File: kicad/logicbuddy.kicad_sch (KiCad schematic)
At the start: 33 parts, among them J1 USB_C_2PIN, Q1 NPN, Q2 NPN, Q3 NPN, Q4 NPN, Q5 NPN, Q6 NPN, Q7 NPN, SW1 SW_SPST, SW2 SW_SPST, SW3 SW_SPST, SW4 SW_SPST, SW5 SW_SPST, SW6 SW_SPST, SW7 SW_SPST, SW8 SW_DIP_x01

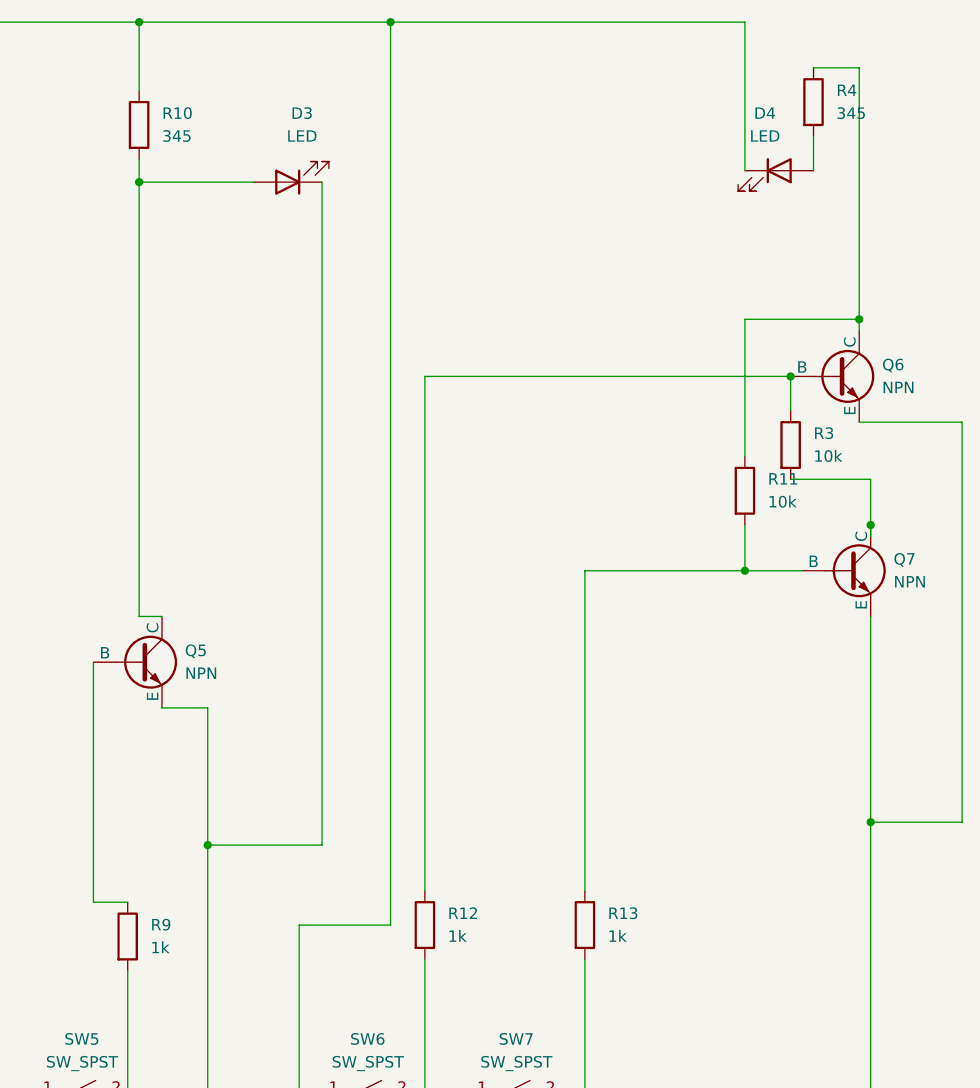
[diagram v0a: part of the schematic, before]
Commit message: Reapply "updated labels and fixed footprints"
This reverts commit 2a946a7896d612220efc5a586cb72ca7f3163489.
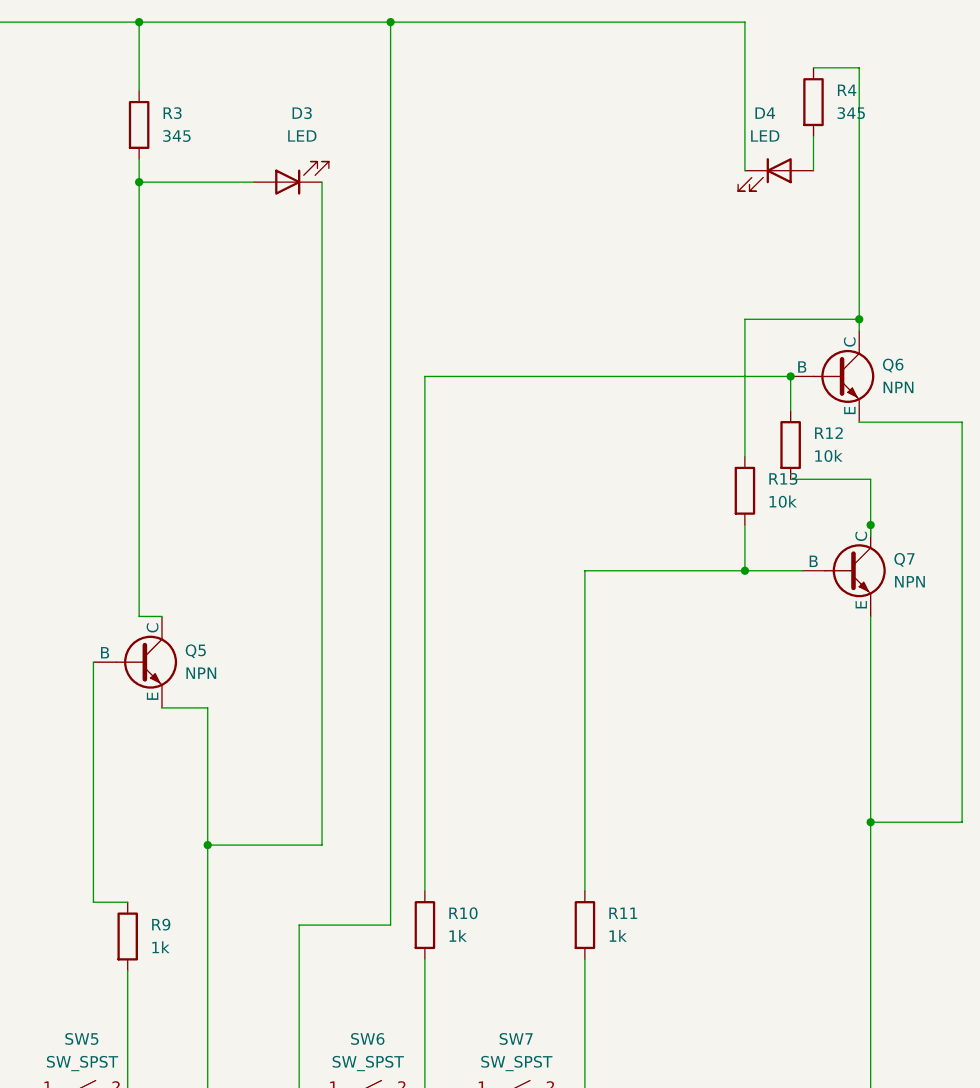
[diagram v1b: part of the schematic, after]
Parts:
- J1: footprint Connector_USB:USB_C_Receptacle_G-Switch_GT-USB-7010ASV -> Aliexpress crap:USB_C_2pin-aliexpress
- SW1, SW2, SW3, SW4, SW5, SW6, SW7: footprint Button_Switch_THT:SW_Push_2P1T_Toggle_CK_PVA1xxH1xxxxxxV2 -> Button_Switch_THT:SW_PUSH_6mm_H5mm
- renumbered R12 to R10, R13 to R11, R3 to R12, R11 to R13, R10 to R3
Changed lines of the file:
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@@
 			)
 		)
-		(property "Footprint" "Button_Switch_THT:SW_Push_2P1T_Toggle_CK_PVA1xxH1xxxxxxV2"
+		(property "Footprint" "Button_Switch_THT:SW_PUSH_6mm_H5mm"
 			(at 92.71 140.97 0)
 			(effects
@@
 			)
 		)
-		(property "Footprint" "Button_Switch_THT:SW_Push_2P1T_Toggle_CK_PVA1xxH1xxxxxxV2"
+		(property "Footprint" "Button_Switch_THT:SW_PUSH_6mm_H5mm"
 			(at 118.11 140.97 0)
 			(effects
@@
 		(dnp no)
 		(fields_autoplaced yes)
-		(property "Reference" "R3"
+		(property "Reference" "R12"
 			(at 234.95 67.3099 0)
 			(effects
@@
 			(project ""
 				(path "/3781676b-6fe7-418a-9d16-7dd26fe4a4bc"
-					(reference "R3")
+					(reference "R12")
 					(unit 1)
 				)
@@
 		(dnp no)
 		(fields_autoplaced yes)
-		(property "Reference" "R12"
+		(property "Reference" "R10"
 			(at 194.31 120.6499 0)
 			(effects
@@
 			(project ""
 				(path "/3781676b-6fe7-418a-9d16-7dd26fe4a4bc"
-					(reference "R12")
+					(reference "R10")
 					(unit 1)
 				)
@@
 			)
 		)
-		(property "Footprint" "Button_Switch_THT:SW_Push_2P1T_Toggle_CK_PVA1xxH1xxxxxxV2"
+		(property "Footprint" "Button_Switch_THT:SW_PUSH_6mm_H5mm"
 			(at 63.5 142.24 0)
 			(effects
@@
 			)
 		)
-		(property "Footprint" "Connector_USB:USB_C_Receptacle_G-Switch_GT-USB-7010ASV"
+		(property "Footprint" "Aliexpress crap:USB_C_2pin-aliexpress"
 			(at 53.34 171.45 0)
 			(effects
@@
 			)
 		)
-		(property "Footprint" "Button_Switch_THT:SW_Push_2P1T_Toggle_CK_PVA1xxH1xxxxxxV2"
+		(property "Footprint" "Button_Switch_THT:SW_PUSH_6mm_H5mm"
 			(at 36.83 142.24 0)
 			(effects
@@
 			)
 		)
-		(property "Footprint" "Button_Switch_THT:SW_Push_2P1T_Toggle_CK_PVA1xxH1xxxxxxV2"
+		(property "Footprint" "Button_Switch_THT:SW_PUSH_6mm_H5mm"
 			(at 201.93 140.97 0)
 			(effects
@@
 			)
 		)
-		(property "Footprint" "Button_Switch_THT:SW_Push_2P1T_Toggle_CK_PVA1xxH1xxxxxxV2"
+		(property "Footprint" "Button_Switch_THT:SW_PUSH_6mm_H5mm"
 			(at 185.42 140.97 0)
 			(effects
@@
 		(dnp no)
 		(fields_autoplaced yes)
-		(property "Reference" "R11"
+		(property "Reference" "R13"
 			(at 229.87 72.3899 0)
 			(effects
@@
 			(project ""
 				(path "/3781676b-6fe7-418a-9d16-7dd26fe4a4bc"
-					(reference "R11")
+					(reference "R13")
 					(unit 1)
 				)
@@
 		(dnp no)
 		(fields_autoplaced yes)
-		(property "Reference" "R10"
+		(property "Reference" "R3"
 			(at 162.56 31.7499 0)
 			(effects
@@
 			(project ""
 				(path "/3781676b-6fe7-418a-9d16-7dd26fe4a4bc"
-					(reference "R10")
+					(reference "R3")
 					(unit 1)
 				)
@@
 		(dnp no)
 		(fields_autoplaced yes)
-		(property "Reference" "R13"
+		(property "Reference" "R11"
 			(at 212.09 120.6499 0)
 			(effects
@@
 			(project ""
 				(path "/3781676b-6fe7-418a-9d16-7dd26fe4a4bc"
-					(reference "R13")
+					(reference "R11")
 					(unit 1)
 				)
@@
 			)
 		)
-		(property "Footprint" "Button_Switch_THT:SW_Push_2P1T_Toggle_CK_PVA1xxH1xxxxxxV2"
+		(property "Footprint" "Button_Switch_THT:SW_PUSH_6mm_H5mm"
 			(at 153.67 140.97 0)
 			(effects

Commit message: Revert "updated labels and fixed footprints"
This reverts commit cc8675b157493e85bb3edc9923989f4c8e1865eb.
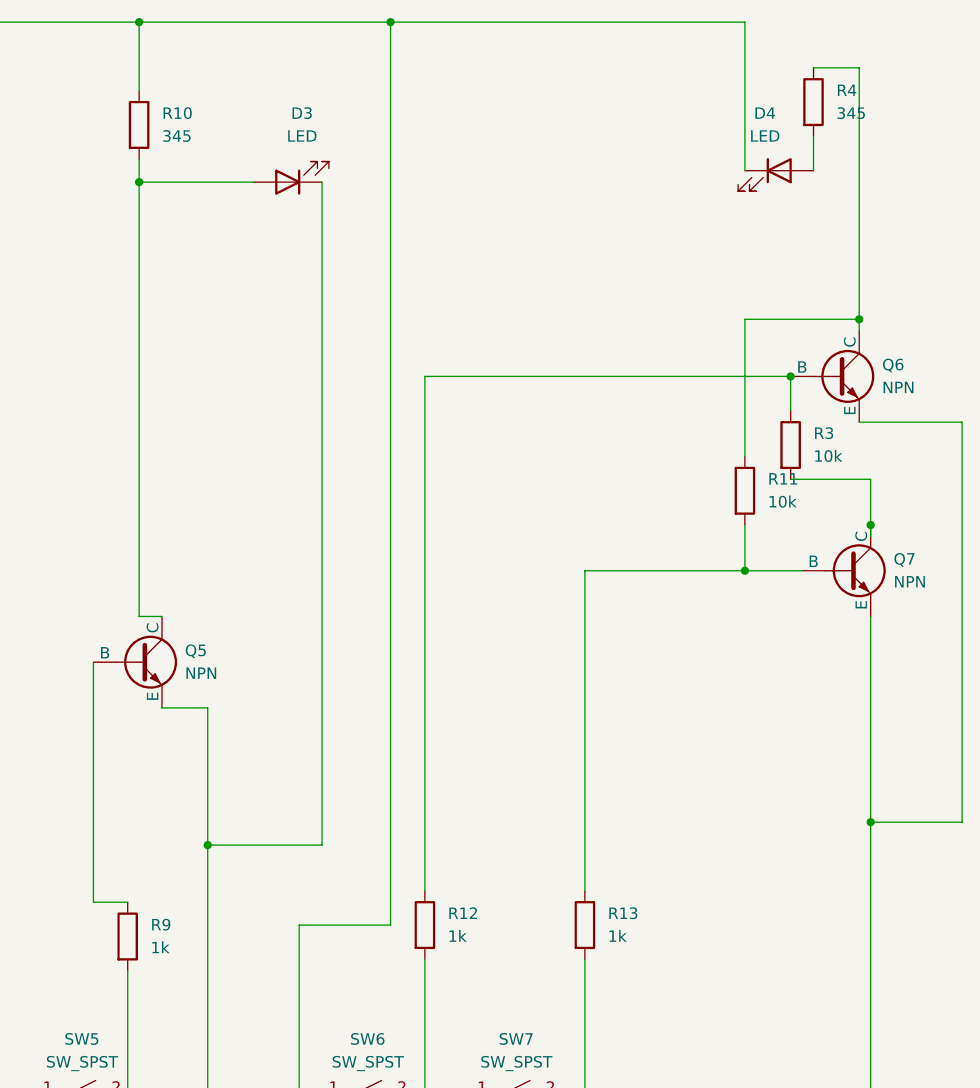
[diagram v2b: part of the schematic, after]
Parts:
- J1: footprint Aliexpress crap:USB_C_2pin-aliexpress -> Connector_USB:USB_C_Receptacle_G-Switch_GT-USB-7010ASV
- SW1, SW2, SW3, SW4, SW5, SW6, SW7: footprint Button_Switch_THT:SW_PUSH_6mm_H5mm -> Button_Switch_THT:SW_Push_2P1T_Toggle_CK_PVA1xxH1xxxxxxV2
- renumbered R3 to R10, R13 to R11, R10 to R12, R11 to R13, R12 to R3
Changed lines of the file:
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@@
 			)
 		)
-		(property "Footprint" "Button_Switch_THT:SW_PUSH_6mm_H5mm"
+		(property "Footprint" "Button_Switch_THT:SW_Push_2P1T_Toggle_CK_PVA1xxH1xxxxxxV2"
 			(at 92.71 140.97 0)
 			(effects
@@
 			)
 		)
-		(property "Footprint" "Button_Switch_THT:SW_PUSH_6mm_H5mm"
+		(property "Footprint" "Button_Switch_THT:SW_Push_2P1T_Toggle_CK_PVA1xxH1xxxxxxV2"
 			(at 118.11 140.97 0)
 			(effects
@@
 		(dnp no)
 		(fields_autoplaced yes)
-		(property "Reference" "R12"
+		(property "Reference" "R3"
 			(at 234.95 67.3099 0)
 			(effects
@@
 			(project ""
 				(path "/3781676b-6fe7-418a-9d16-7dd26fe4a4bc"
-					(reference "R12")
+					(reference "R3")
 					(unit 1)
 				)
@@
 		(dnp no)
 		(fields_autoplaced yes)
-		(property "Reference" "R10"
+		(property "Reference" "R12"
 			(at 194.31 120.6499 0)
 			(effects
@@
 			(project ""
 				(path "/3781676b-6fe7-418a-9d16-7dd26fe4a4bc"
-					(reference "R10")
+					(reference "R12")
 					(unit 1)
 				)
@@
 			)
 		)
-		(property "Footprint" "Button_Switch_THT:SW_PUSH_6mm_H5mm"
+		(property "Footprint" "Button_Switch_THT:SW_Push_2P1T_Toggle_CK_PVA1xxH1xxxxxxV2"
 			(at 63.5 142.24 0)
 			(effects
@@
 			)
 		)
-		(property "Footprint" "Aliexpress crap:USB_C_2pin-aliexpress"
+		(property "Footprint" "Connector_USB:USB_C_Receptacle_G-Switch_GT-USB-7010ASV"
 			(at 53.34 171.45 0)
 			(effects
@@
 			)
 		)
-		(property "Footprint" "Button_Switch_THT:SW_PUSH_6mm_H5mm"
+		(property "Footprint" "Button_Switch_THT:SW_Push_2P1T_Toggle_CK_PVA1xxH1xxxxxxV2"
 			(at 36.83 142.24 0)
 			(effects
@@
 			)
 		)
-		(property "Footprint" "Button_Switch_THT:SW_PUSH_6mm_H5mm"
+		(property "Footprint" "Button_Switch_THT:SW_Push_2P1T_Toggle_CK_PVA1xxH1xxxxxxV2"
 			(at 201.93 140.97 0)
 			(effects
@@
 			)
 		)
-		(property "Footprint" "Button_Switch_THT:SW_PUSH_6mm_H5mm"
+		(property "Footprint" "Button_Switch_THT:SW_Push_2P1T_Toggle_CK_PVA1xxH1xxxxxxV2"
 			(at 185.42 140.97 0)
 			(effects
@@
 		(dnp no)
 		(fields_autoplaced yes)
-		(property "Reference" "R13"
+		(property "Reference" "R11"
 			(at 229.87 72.3899 0)
 			(effects
@@
 			(project ""
 				(path "/3781676b-6fe7-418a-9d16-7dd26fe4a4bc"
-					(reference "R13")
+					(reference "R11")
 					(unit 1)
 				)
@@
 		(dnp no)
 		(fields_autoplaced yes)
-		(property "Reference" "R3"
+		(property "Reference" "R10"
 			(at 162.56 31.7499 0)
 			(effects
@@
 			(project ""
 				(path "/3781676b-6fe7-418a-9d16-7dd26fe4a4bc"
-					(reference "R3")
+					(reference "R10")
 					(unit 1)
 				)
@@
 		(dnp no)
 		(fields_autoplaced yes)
-		(property "Reference" "R11"
+		(property "Reference" "R13"
 			(at 212.09 120.6499 0)
 			(effects
@@
 			(project ""
 				(path "/3781676b-6fe7-418a-9d16-7dd26fe4a4bc"
-					(reference "R11")
+					(reference "R13")
 					(unit 1)
 				)
@@
 			)
 		)
-		(property "Footprint" "Button_Switch_THT:SW_PUSH_6mm_H5mm"
+		(property "Footprint" "Button_Switch_THT:SW_Push_2P1T_Toggle_CK_PVA1xxH1xxxxxxV2"
 			(at 153.67 140.97 0)
 			(effects
